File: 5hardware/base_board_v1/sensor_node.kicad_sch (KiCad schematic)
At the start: 21 parts, among them J1 Conn_01x06_Pin, J2 Conn_01x08_Pin, J3 Conn_01x09_Pin, J4 USB_C_Receptacle_USB2.0, P1 USB_C_Plug_USB2.0, SW1 SW_Push, SW2 SW_Push, SW7 SW_Push, U1 ESP-12F, U2 CH32V003F4P6, U3 XC6206PxxxMR

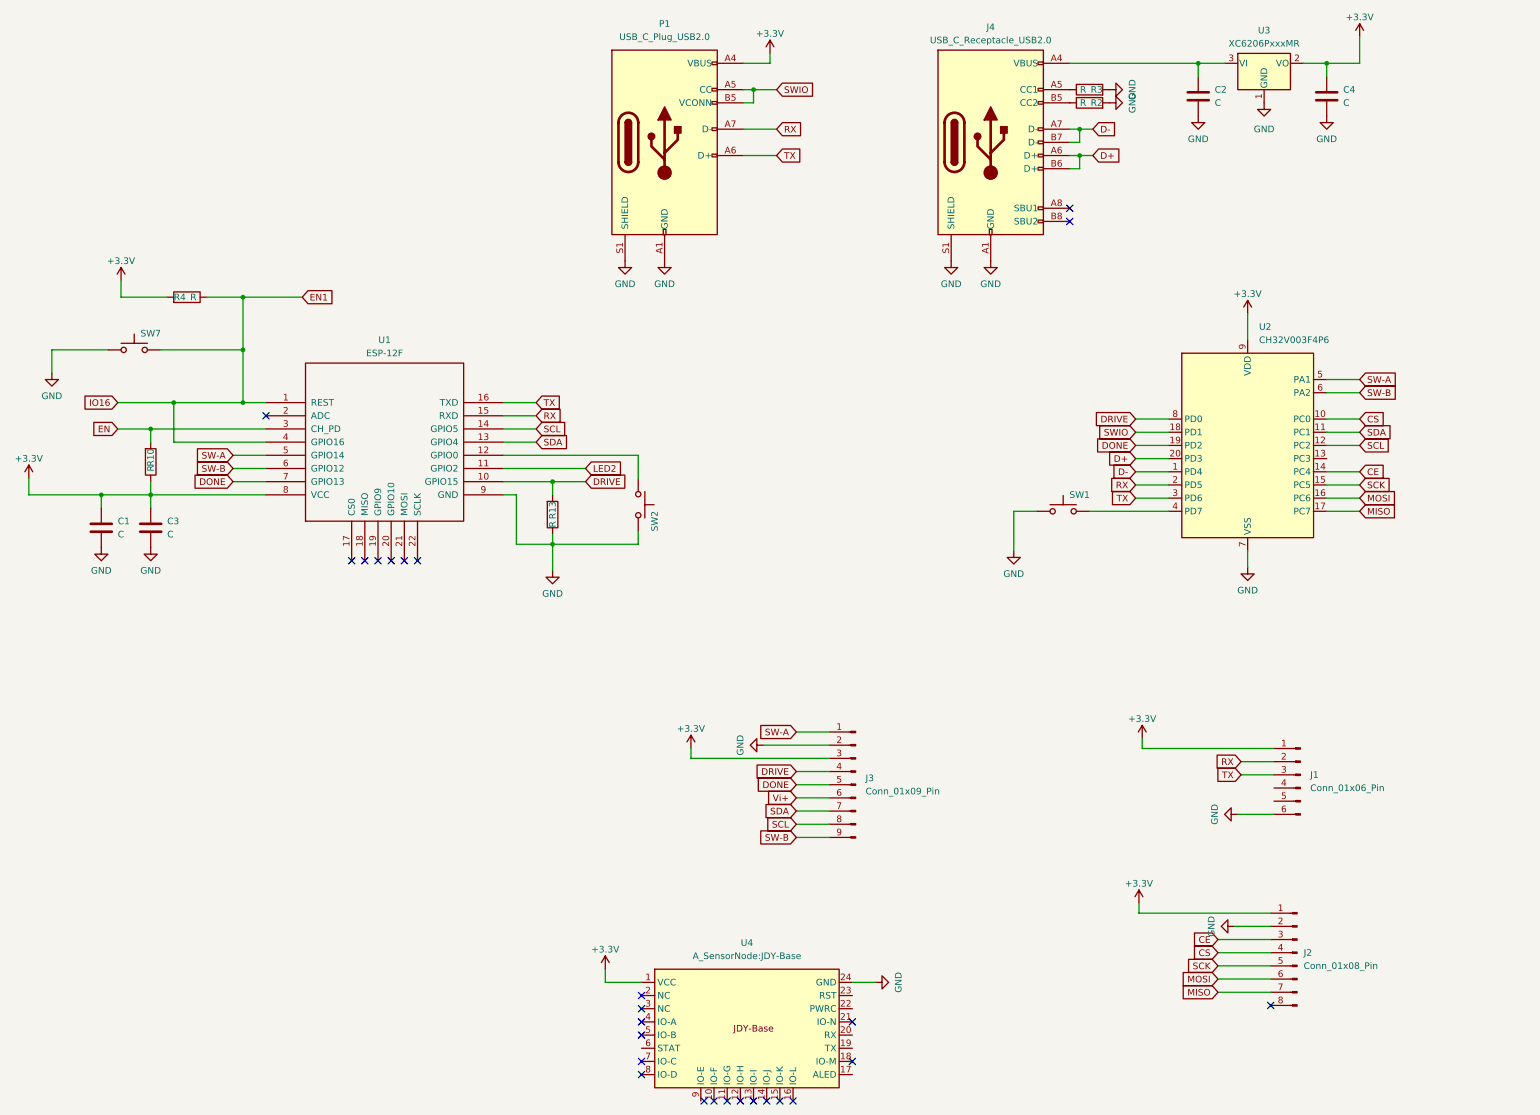
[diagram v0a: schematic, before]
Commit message: update pcb.
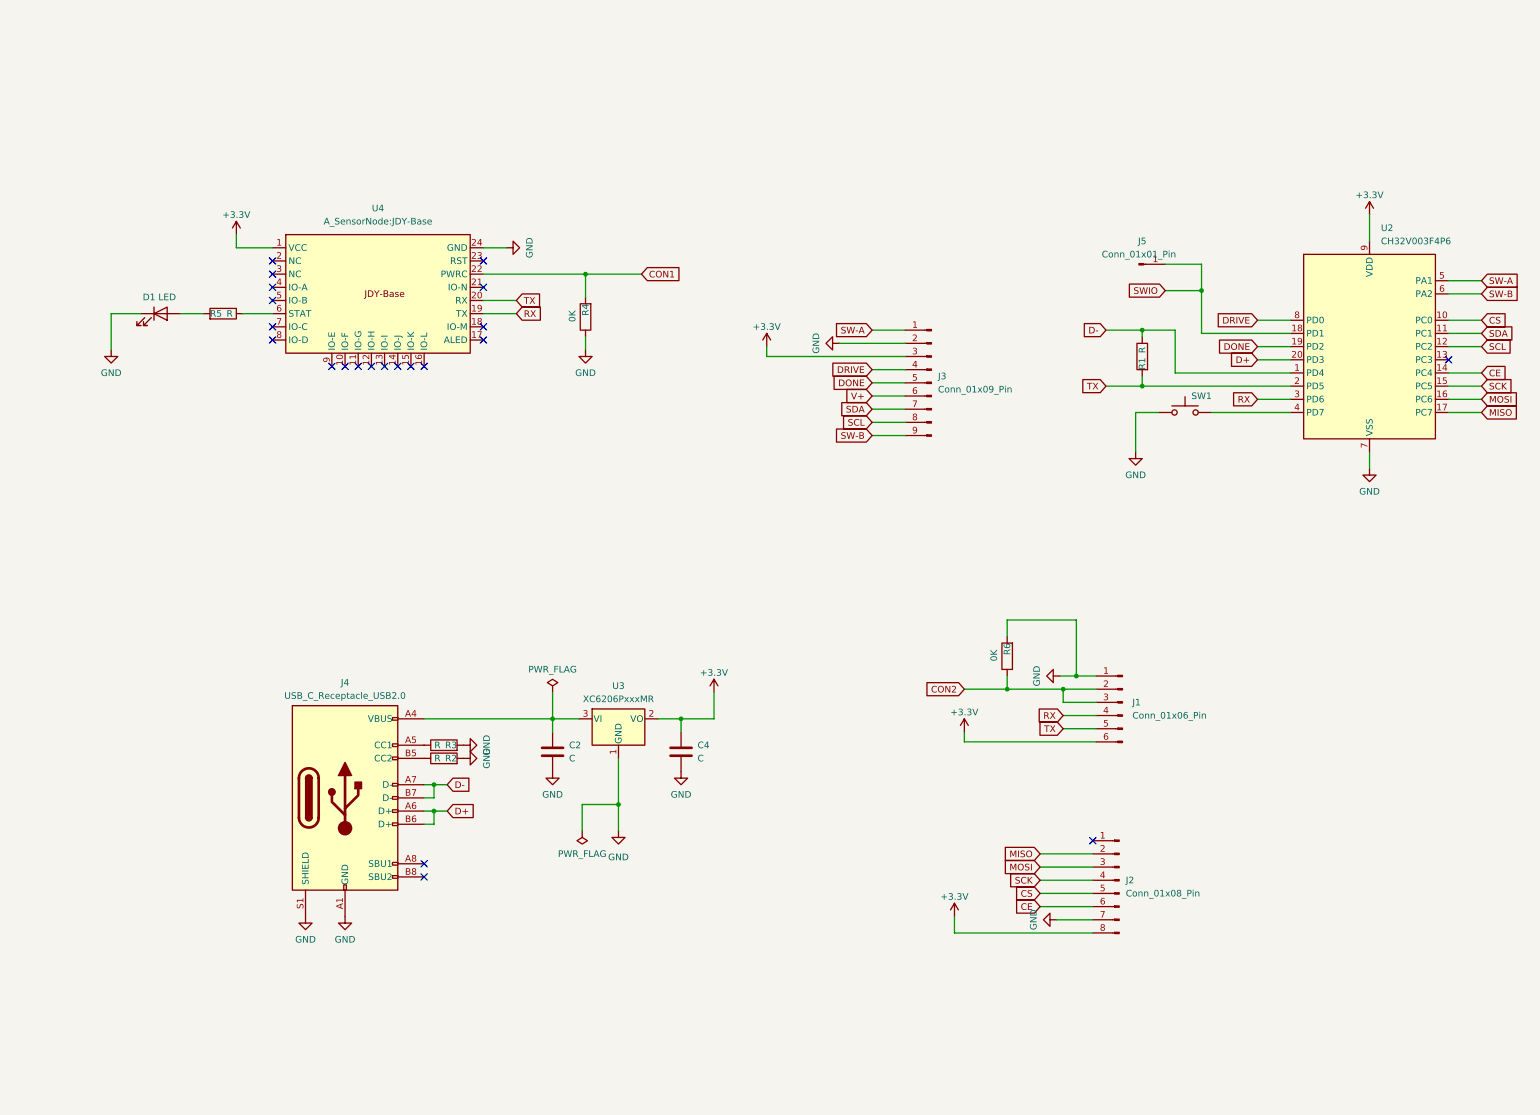
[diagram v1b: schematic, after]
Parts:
- removed C1, C3: C, Capacitor_SMD:C_0603_1608Metric, symbol Device:C
- removed P1: USB_C_Plug_USB2.0, Connector_USB:USB_C_Receptacle_GCT_USB4135-GF-A_6P_TopMnt_Horizontal, symbol Connector:USB_C_Plug_USB2.0
- removed R10, R13: R, Resistor_SMD:R_0603_1608Metric, symbol Device:R
- removed SW2, SW7: SW_Push, Button_Switch_SMD:SW_SPST_PTS810, symbol Switch:SW_Push
- removed U1: ESP-12F, A_SensorNode:ESP12_SMD, symbol ESP8266:ESP-12F
- added D1: LED, LED_SMD:LED_0603_1608Metric, symbol Device:LED
- added J5: Conn_01x01_Pin, Connector_PinHeader_2.54mm:PinHeader_1x01_P2.54mm_Vertical, symbol Connector:Conn_01x01_Pin
- added R1, R5: R, Resistor_SMD:R_0603_1608Metric, symbol Device:R
- added R6: 0K, A_SensorNode:Jumpper, symbol Device:R
- J4: footprint Connector_USB:USB_C_Receptacle_GCT_USB4105-xx-A_16P_TopMnt_Horizontal -> Connector_USB:USB_C_Receptacle_HRO_TYPE-C-31-M-12
- R4: value R -> 0K; footprint Resistor_SMD:R_0603_1608Metric -> A_SensorNode:Jumpper
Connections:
- net EN1 is gone; now on net GND: R4.1
- net +3.3V: now also J1.6 (Pin_6), J2.8 (Pin_8); no longer J1.1 (Pin_1), J2.1 (Pin_1), R4.2
- net CE: now also J2.6 (Pin_6); no longer J2.3 (Pin_3)
- net CS: now also J2.5 (Pin_5); no longer J2.4 (Pin_4)
- net D-: now also R1.1
- net GND: now also J1.1 (Pin_1), J2.7 (Pin_7), D1.1 (K), R6.2; no longer J1.6 (Pin_6), J2.2 (Pin_2)
- net MISO: now also J2.2 (Pin_2); no longer J2.7 (Pin_7)
- net MOSI: now also J2.3 (Pin_3); no longer J2.6 (Pin_6)
- net RX: now also J1.4 (Pin_4), U2.3 (PD6), U4.19 (TX); no longer J1.2 (Pin_2), U2.2 (PD5)
- net SCK: now also J2.4 (Pin_4); no longer J2.5 (Pin_5)
- net SWIO: now also J5.1 (Pin_1)
- net TX: now also J1.5 (Pin_5), U2.2 (PD5), U4.20 (RX), R1.2; no longer J1.3 (Pin_3), U2.3 (PD6)
- net CON1: now reaches U4.22 (PWRC)
- net CON1: now also R4.2
- net at U4.6 (STAT): now also R5.1
- net Vi+ renamed V+
- new net: D1.2 (A), R5.2
- new net CON2: J1.2 (Pin_2), J1.3 (Pin_3), R6.1
- no-connect marks 26 -> 22
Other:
- moved on the sheet: C2, C4, J1, J2, J4, R2, R3, SW1, U2, U3, U4
